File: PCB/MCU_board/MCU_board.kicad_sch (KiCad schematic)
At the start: 9 parts, among them IC3 ESP32-S3-WROOM-1-N4R8, J1 DS1013-40SSIB1-B-0

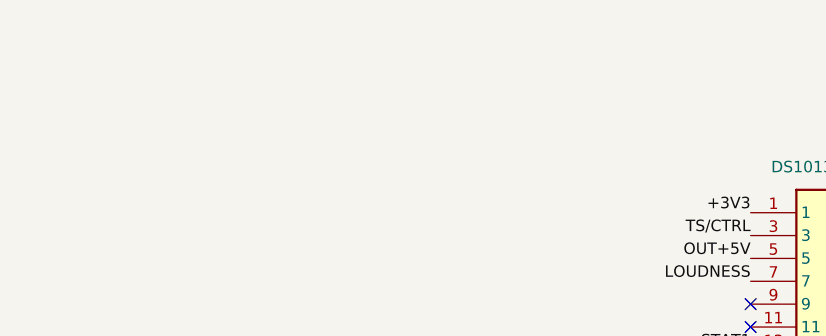
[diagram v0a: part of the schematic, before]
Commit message: everything checked
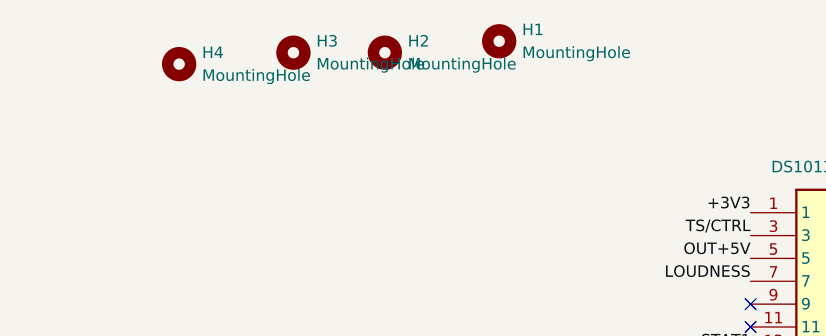
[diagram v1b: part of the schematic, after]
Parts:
- added H1, H2, H3, H4: MountingHole, MountingHole:MountingHole_3.2mm_M3_Pad_Via, symbol Mechanical:MountingHole
